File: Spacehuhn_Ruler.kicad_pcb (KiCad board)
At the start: 2 copper layers, 150 x 25.4 mm, 47 parts

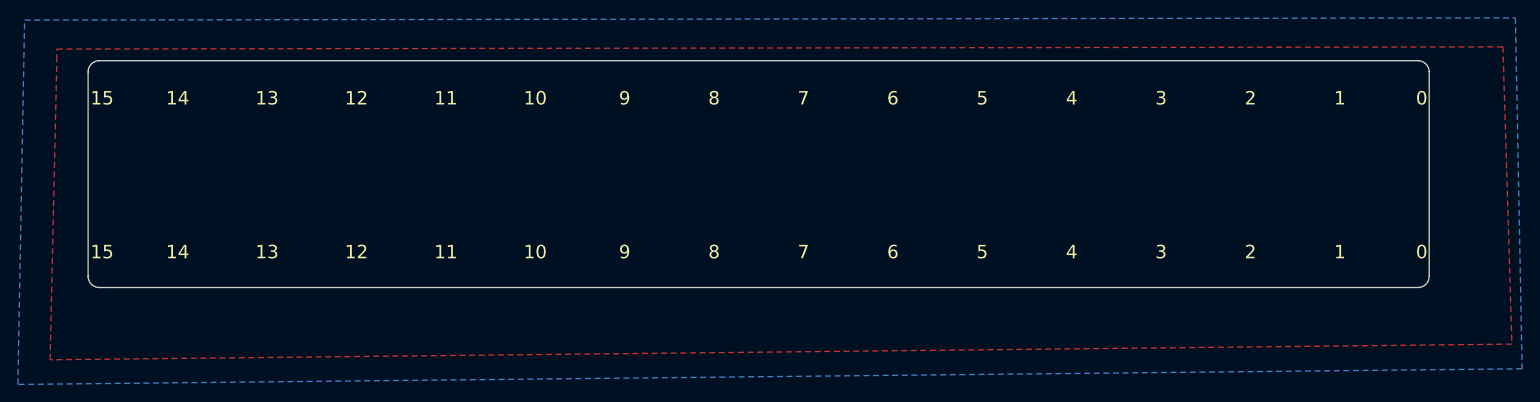
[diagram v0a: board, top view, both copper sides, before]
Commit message: Cleanup
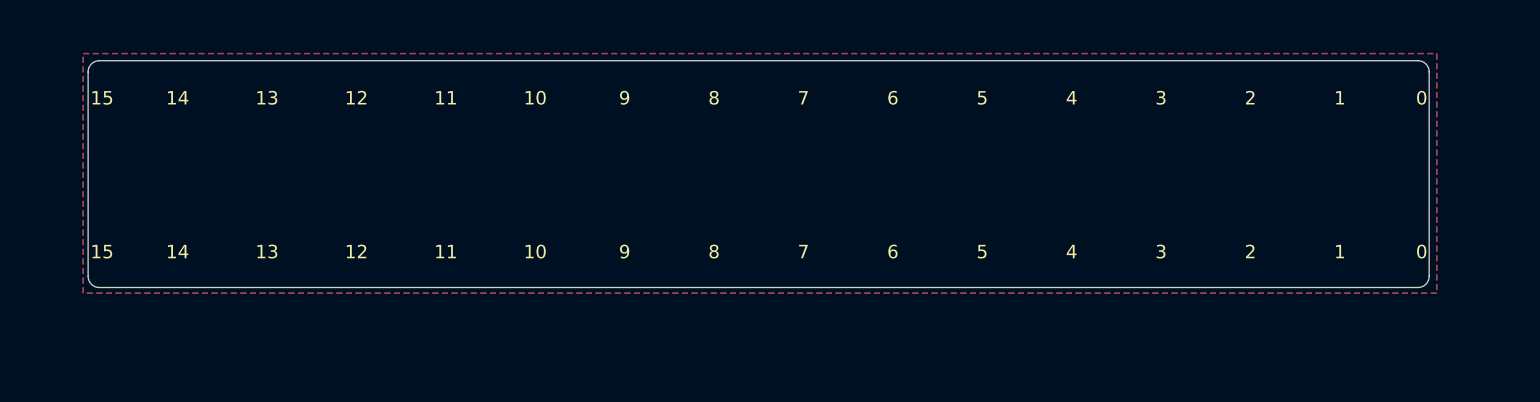
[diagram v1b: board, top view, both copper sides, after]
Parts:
- G*** (x2): footprint PCB-Art:blackhole -> Artwork:blackhole-mask
- G*** (x2): footprint PCB-Art:comet -> Artwork:comet-mask
- G*** (x6): footprint PCB-Art:star3 -> Artwork:star3-mask
- G*** (x2): footprint PCB-Art:planet2 -> Artwork:planet2-mask
- G*** (x13): footprint PCB-Art:star1 -> Artwork:star1-mask
- G*** (x2): footprint PCB-Art:spaceship -> Artwork:spaceship-mask
- G*** (x10): footprint PCB-Art:star2 -> Artwork:star2-mask
- G*** (x2): footprint PCB-Art:planet -> Artwork:planet-mask
- G*** (x2): footprint PCB-Art:spacehuhn_text -> Artwork:spacehuhn_text-mask
- G*** (x2): footprint PCB-Art:spacehuhn -> Artwork:spacehuhn-mask
- G*** (x2): footprint PCB-Art:bigdipper -> Artwork:bigdipper-mask
- G*** (x2): footprint PCB-Art:galaxy1 -> Artwork:galaxy1-mask
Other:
- board text added: "1 inch"
- board text added: "5.9 inch"
- board text removed: "it 1 inch lol"
- board text removed: "rev2"
